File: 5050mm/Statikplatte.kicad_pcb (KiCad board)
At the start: 4 copper layers, 50 x 50 mm, 23 parts, among them J10 HV, J2 GND, J3 IN+, J4 GND, J5 GND, J6 GND, J7 HV, J8 HV, J9 HV

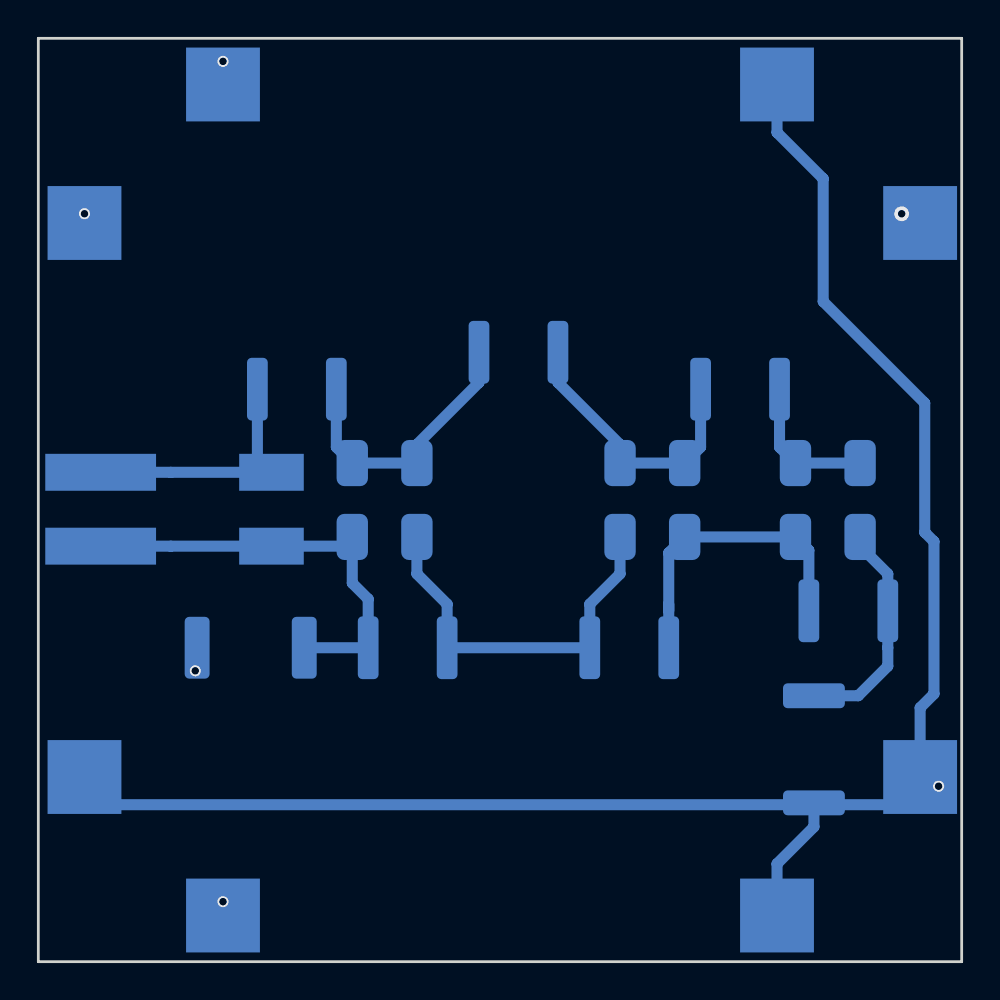
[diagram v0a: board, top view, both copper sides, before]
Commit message: updated to KICAD 6
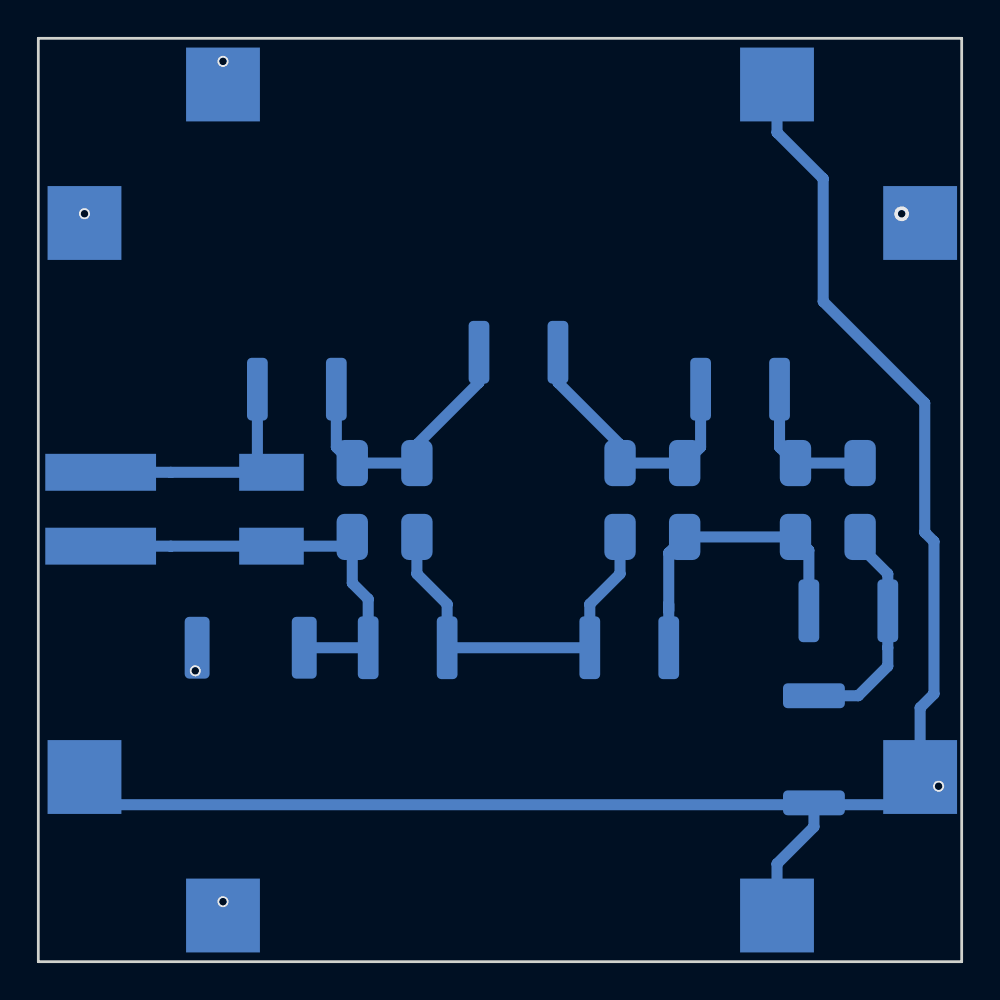
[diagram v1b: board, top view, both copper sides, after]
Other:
- net class Default removed
